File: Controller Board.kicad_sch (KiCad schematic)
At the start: 3 parts, among them J1 Conn_01x12_Socket, J2 Conn_01x12_Socket

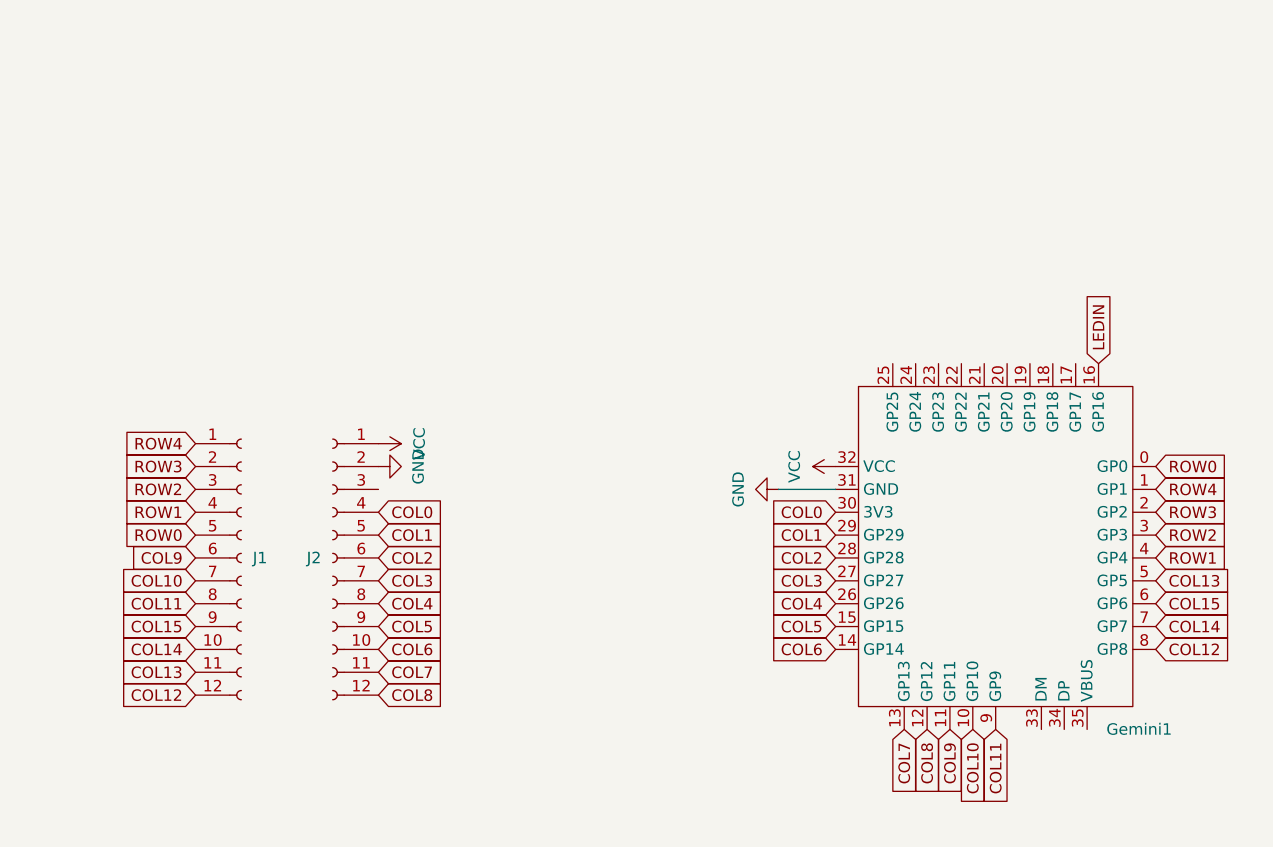
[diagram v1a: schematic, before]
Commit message: checkpoint
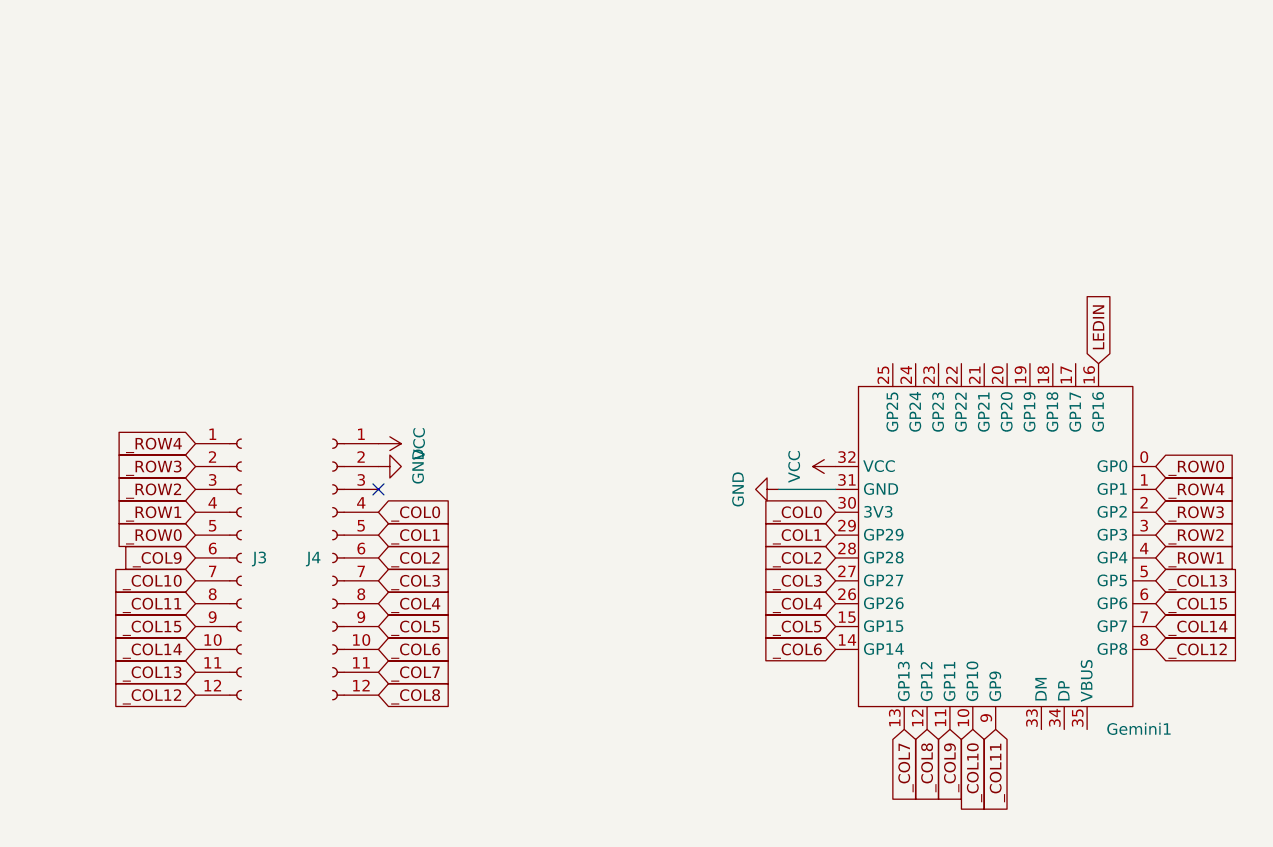
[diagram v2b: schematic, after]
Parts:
- J3: renamed from J1; value Conn_01x12_Socket -> Conn_01x12_Header; footprint Connector_PinSocket_2.54mm:PinSocket_1x12_P2.54mm_Vertical -> Connector_PinHeader_2.54mm:PinHeader_1x12_P2.54mm_Vertical
- J4: renamed from J2; value Conn_01x12_Socket -> Conn_01x12_Header; footprint Connector_PinSocket_2.54mm:PinSocket_1x12_P2.54mm_Vertical -> Connector_PinHeader_2.54mm:PinHeader_1x12_P2.54mm_Vertical
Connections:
- net COL0 renamed _COL0
- net COL1 renamed _COL1
- net COL10 renamed _COL10
- net COL11 renamed _COL11
- net COL12 renamed _COL12
- net COL13 renamed _COL13
- net COL14 renamed _COL14
- net COL15 renamed _COL15
- net COL2 renamed _COL2
- net COL3 renamed _COL3
- net COL4 renamed _COL4
- net COL5 renamed _COL5
- net COL6 renamed _COL6
- net COL7 renamed _COL7
- net COL8 renamed _COL8
- net COL9 renamed _COL9
- net ROW0 renamed _ROW0
- net ROW1 renamed _ROW1
- net ROW2 renamed _ROW2
- net ROW3 renamed _ROW3
- net ROW4 renamed _ROW4
- no-connect marks 0 -> 1

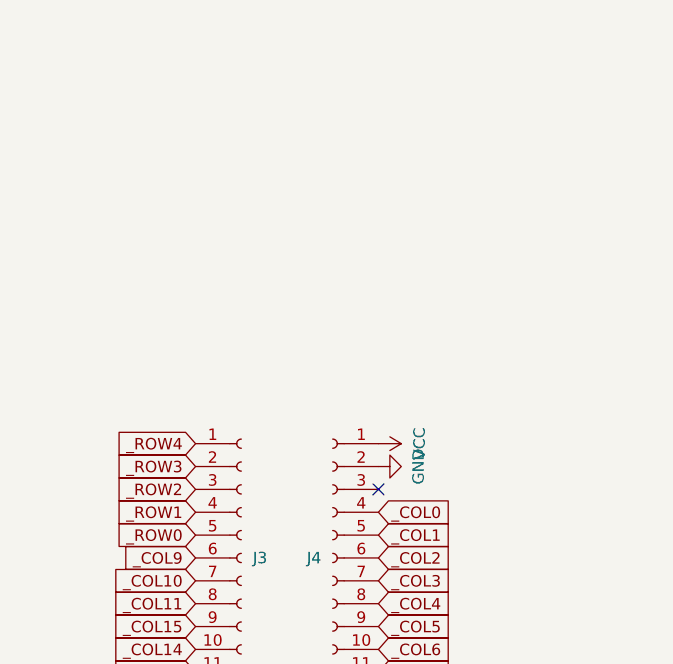
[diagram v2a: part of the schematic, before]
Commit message: checkpoint w gemini routed
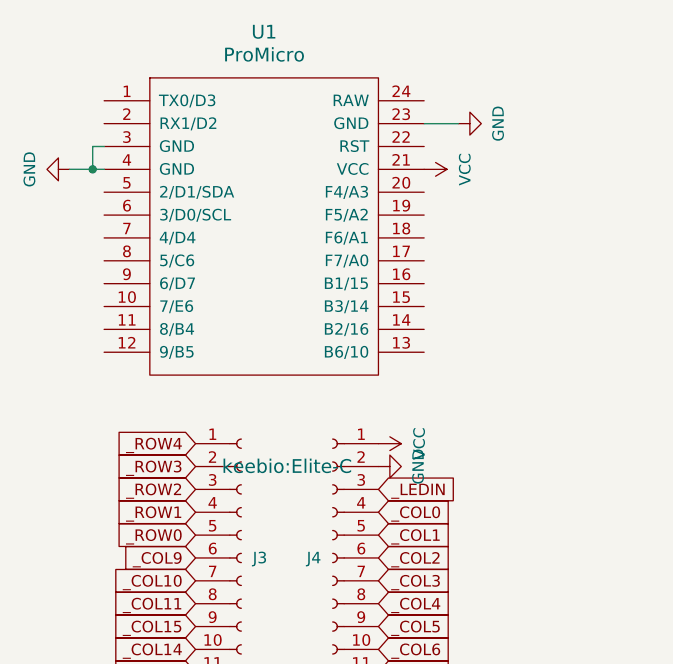
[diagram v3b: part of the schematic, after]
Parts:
- added U1: ProMicro, keebio:Elite-C, symbol kbd:ProMicro
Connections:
- net GND: now also U1.23 (GND), U1.3 (GND), U1.4 (GND)
- net VCC: now also U1.21 (VCC)
- net _LEDIN: now reaches J4.3 (Pin_3)
- no-connect marks 1 -> 0
